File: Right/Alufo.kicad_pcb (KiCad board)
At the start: 2 copper layers, 139.7 x 88.9 mm, 67 parts, among them J2 USB_C_Receptacle_USB2.0_16P_2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, J4 USB_C_Receptacle_USB2.0_16P_2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, K11 PG1350, K12 PG1350, K13 PG1350, K14 PG1350, K15 PG1350, K16 PG1350, K21 PG1350, K22 PG1350, K23 PG1350, K24 PG1350, K25 PG1350, K26 PG1350, K32 PG1350, K33 PG1350, K34 PG1350, K35 PG1350, K41 PG1350_1½U, K42 PG1350/SKQUCAA010, SW2 BOOT, U2 CH552T, U4 USBLC6-2P6, U6 USBLC6-2P6

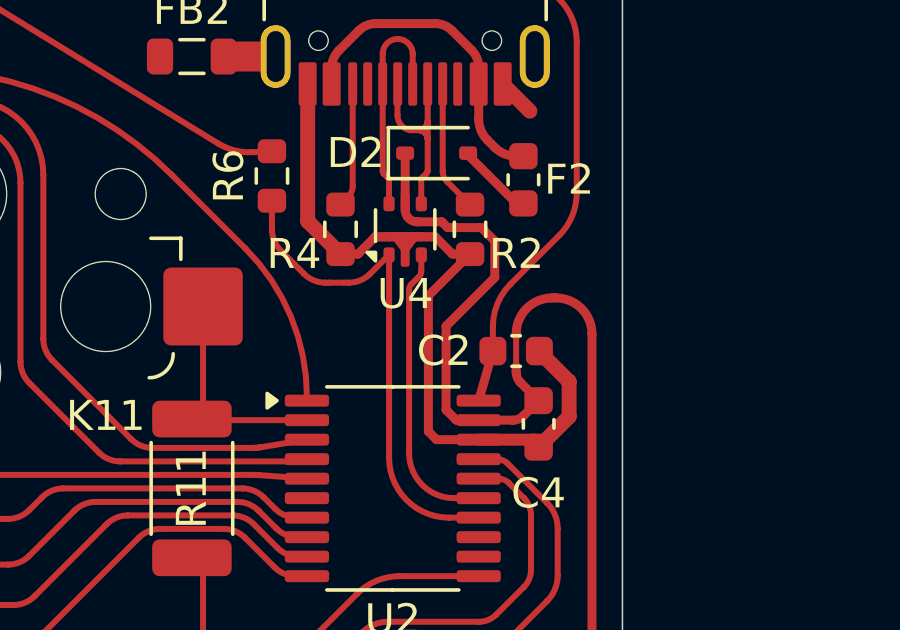
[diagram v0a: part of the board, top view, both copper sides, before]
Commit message: Minor tweaks
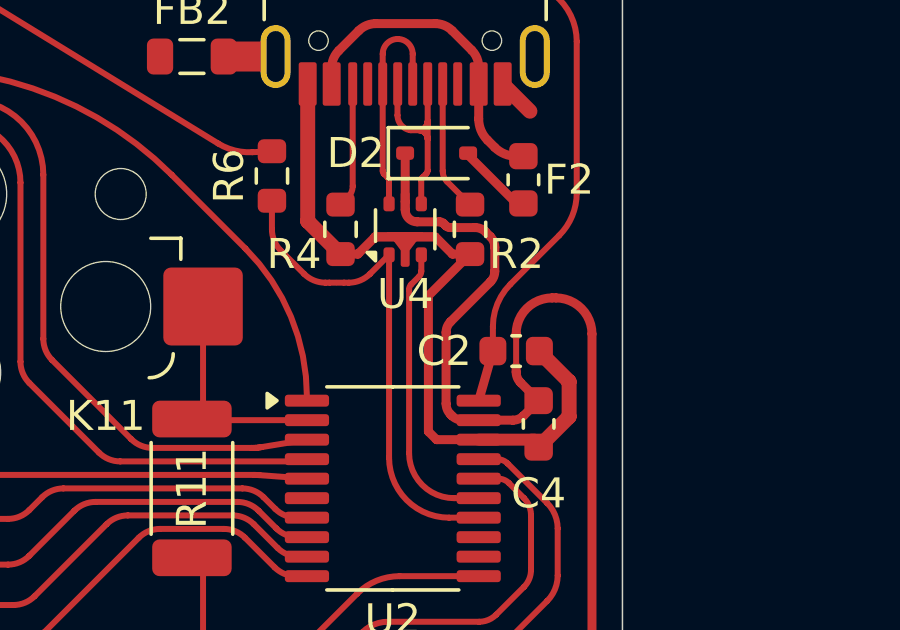
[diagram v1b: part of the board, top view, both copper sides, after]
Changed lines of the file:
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@@
-	)
-	(segment
-		(start 215.408 53.344008)
-		(end 216.23265 53.344008)
-		(width 0.3)
-		(layer "F.Cu")
-		(net 21)
-	)
-	(segment
-		(start 216.7144 59.955)
-		(end 216.8705 59.955)
-		(width 0.3)
-		(layer "F.Cu")
-		(net 21)
 	)
 	(segment
@@
 	)
 	(segment
-		(start 216.23265 53.344008)
-		(end 216.424064 53.535422)
-		(width 0.3)
-		(layer "F.Cu")
-		(net 21)
-	)
-	(segment
 		(start 215.722315 71.450999)
 		(end 216.300686 72.02937)
@@
 		(start 212.074 71.882)
 		(end 212.074 71.464344)
-		(width 0.3)
-		(layer "F.Cu")
-		(net 21)
-	)
-	(segment
-		(start 216.424064 53.535422)
-		(end 217.54478 53.535422)
 		(width 0.3)
 		(layer "F.Cu")
@@
 	)
 	(segment
+		(start 216.506907 53.535422)
+		(end 217.337673 53.535422)
+		(width 0.3)
+		(layer "F.Cu")
+		(net 21)
+	)
+	(segment
+		(start 217.691227 53.681869)
+		(end 217.848554 53.839196)
+		(width 0.3)
+		(layer "F.Cu")
+		(net 21)
+	)
+	(segment
+		(start 216.291229 53.402587)
+		(end 216.365486 53.476844)
+		(width 0.3)
+		(layer "F.Cu")
+		(net 21)
+	)
+	(segment
+		(start 218.705999 58.347892)
+		(end 218.705999 58.166)
+		(width 0.3)
+		(layer "F.Cu")
+		(net 21)
+	)
+	(segment
+		(start 216.300685 75.303999)
+		(end 215.722314 75.88237)
+		(width 0.3)
+		(layer "F.Cu")
+		(net 21)
+	)
+	(segment
+		(start 219.905999 55.88)
+		(end 220.034 55.88)
+		(width 0.3)
+		(layer "F.Cu")
+		(net 21)
+	)
+	(segment
+		(start 217.458 59.955)
+		(end 218.598893 59.955)
+		(width 0.3)
+		(layer "F.Cu")
+		(net 21)
+	)
+	(segment
+		(start 217.995 54.192749)
+		(end 217.995 54.991376)
+		(width 0.3)
+		(layer "F.Cu")
+		(net 21)
+	)
+	(segment
+		(start 215.408 53.344008)
+		(end 216.149807 53.344008)
+		(width 0.3)
+		(layer "F.Cu")
+		(net 21)
+	)
+	(segment
+		(start 216.3705 57.03009)
+		(end 216.3705 59.403993)
+		(width 0.3)
+		(layer "F.Cu")
+		(net 21)
+	)
+	(segment
+		(start 216.516947 59.757547)
+		(end 216.567954 59.808554)
+		(width 0.3)
+		(layer "F.Cu")
+		(net 21)
+	)
+	(segment
+		(start 217.848553 55.34493)
+		(end 216.516946 56.676537)
+		(width 0.3)
+		(layer "F.Cu")
+		(net 21)
+	)
+	(segment
+		(start 216.921507 59.955)
+		(end 217.458 59.955)
+		(width 0.3)
+		(layer "F.Cu")
+		(net 21)
+	)
+	(segment
 		(start 215.008 52.669)
 		(end 215.008 52.944008)
-		(width 0.3)
-		(layer "F.Cu")
-		(net 21)
-	)
-	(segment
-		(start 218.705999 58.347892)
-		(end 218.705999 58.166)
-		(width 0.3)
-		(layer "F.Cu")
-		(net 21)
-	)
-	(segment
-		(start 216.300685 75.303999)
-		(end 215.722314 75.88237)
-		(width 0.3)
-		(layer "F.Cu")
-		(net 21)
-	)
-	(segment
-		(start 217.54478 53.535422)
-		(end 217.995 53.985642)
-		(width 0.3)
-		(layer "F.Cu")
-		(net 21)
-	)
-	(segment
-		(start 216.3705 56.822983)
-		(end 216.3705 59.6111)
-		(width 0.3)
-		(layer "F.Cu")
-		(net 21)
-	)
-	(segment
-		(start 216.3705 59.6111)
-		(end 216.7144 59.955)
-		(width 0.3)
-		(layer "F.Cu")
-		(net 21)
-	)
-	(segment
-		(start 217.995 53.985642)
-		(end 217.995 55.198483)
-		(width 0.3)
-		(layer "F.Cu")
-		(net 21)
-	)
-	(segment
-		(start 219.905999 55.88)
-		(end 220.034 55.88)
-		(width 0.3)
-		(layer "F.Cu")
-		(net 21)
-	)
-	(segment
-		(start 217.458 59.955)
-		(end 218.598893 59.955)
-		(width 0.3)
-		(layer "F.Cu")
-		(net 21)
-	)
-	(segment
-		(start 217.995 55.198483)
-		(end 216.3705 56.822983)
 		(width 0.3)
 		(layer "F.Cu")
@@
 	)
 	(arc
+		(start 216.365486 53.476844)
+		(mid 216.430371 53.520198)
+		(end 216.506907 53.535422)
+		(width 0.3)
+		(layer "F.Cu")
+		(net 21)
+	)
+	(arc
 		(start 215.722314 75.88237)
 		(mid 215.462775 76.055788)
@@
 	)
 	(arc
+		(start 216.149807 53.344008)
+		(mid 216.226344 53.359232)
+		(end 216.291229 53.402587)
+		(width 0.3)
+		(layer "F.Cu")
+		(net 21)
+	)
+	(arc
+		(start 217.337673 53.535422)
+		(mid 217.529015 53.573482)
+		(end 217.691227 53.681869)
+		(width 0.3)
+		(layer "F.Cu")
+		(net 21)
+	)
+	(arc
 		(start 216.535 74.738313)
 		(mid 216.474103 75.04446)
@@
 	)
 	(arc
+		(start 216.3705 57.03009)
+		(mid 216.40856 56.838749)
+		(end 216.516946 56.676537)
+		(width 0.3)
+		(layer "F.Cu")
+		(net 21)
+	)
+	(arc
 		(start 216.535 72.595055)
 		(mid 216.474104 72.288909)
@@
 	)
 	(arc
+		(start 217.995 54.991376)
+		(mid 217.95694 55.182718)
+		(end 217.848553 55.34493)
+		(width 0.3)
+		(layer "F.Cu")
+		(net 21)
+	)
+	(arc
+		(start 215.008 52.944008)
+		(mid 215.125157 53.226851)
+		(end 215.408 53.344008)
+		(width 0.3)
+		(layer "F.Cu")
+		(net 21)
+	)
+	(arc
 		(start 218.952447 59.808553)
 		(mid 218.790235 59.91694)
@@
 	)
 	(arc
-		(start 215.408 53.344008)
-		(mid 215.125157 53.226851)
-		(end 215.008 52.944008)
-		(width 0.3)
-		(layer "F.Cu")
+		(start 216.516947 59.757547)
+		(mid 216.40856 59.595335)
+		(end 216.3705 59.403993)
+		(width 0.3)
+		(layer "F.Cu")
+		(net 21)
+	)
+	(arc
+		(start 217.995 54.192749)
+		(mid 217.95694 54.001408)
+		(end 217.848554 53.839196)
+		(width 0.3)
+		(layer "F.Cu")
+		(net 21)
+	)
+	(arc
+		(start 216.567954 59.808554)
+		(mid 216.730166 59.91694)
+		(end 216.921507 59.955)
+		(width 0.3)
+		(layer "F.Cu")

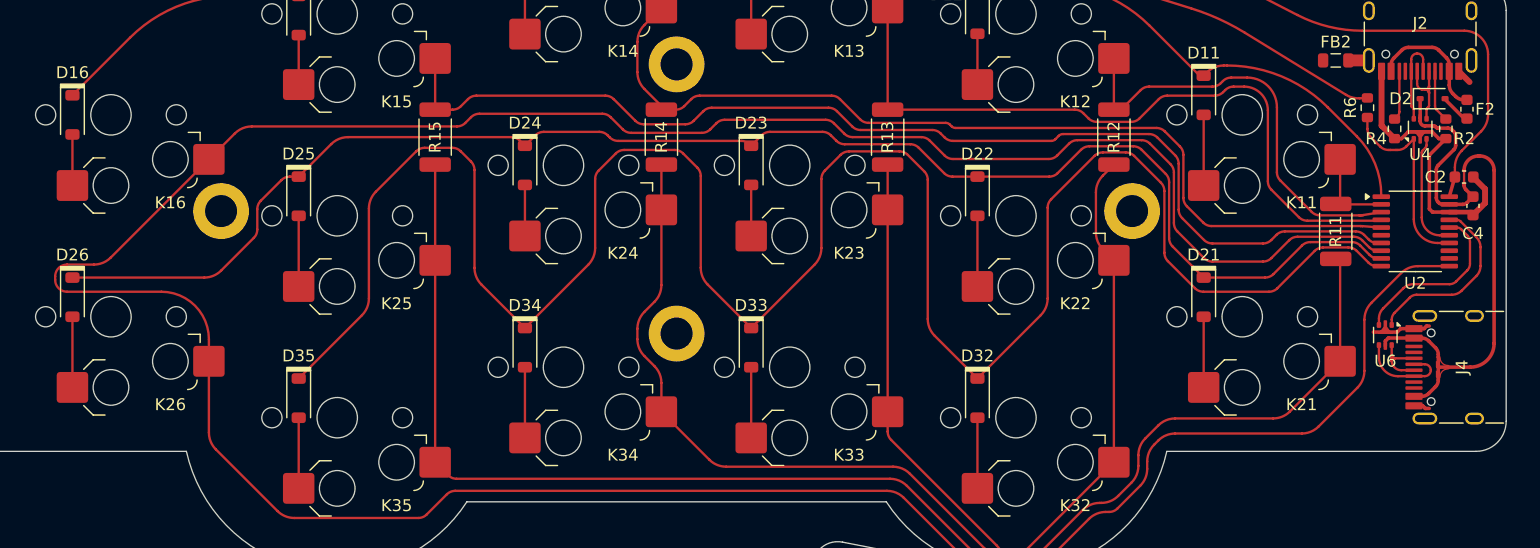
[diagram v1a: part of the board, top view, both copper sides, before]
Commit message: Further routing tweaks
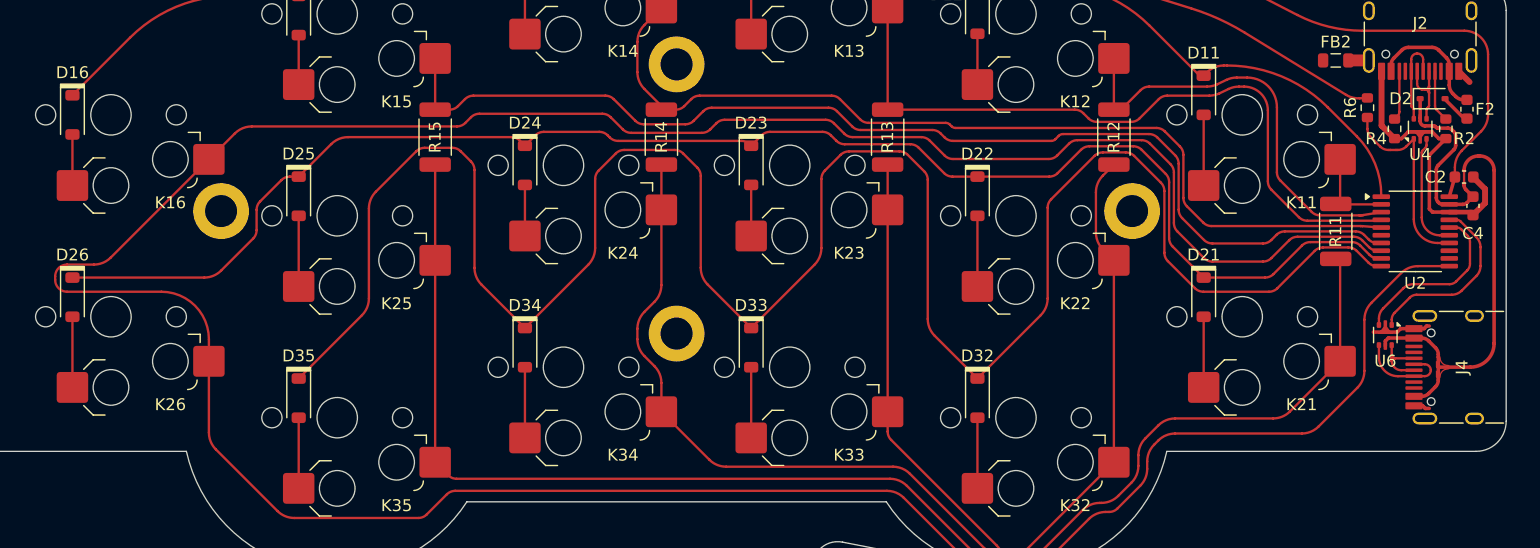
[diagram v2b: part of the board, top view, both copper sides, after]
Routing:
- net Col5T: track 93.5 -> 92.0 mm
- net Col2T: track 62.2 -> 60.8 mm
- net Col4: track 77.6 -> 76.4 mm
- net Col2: track 36.2 -> 35.2 mm
- net VCC: track 52.2 -> 51.6 mm
